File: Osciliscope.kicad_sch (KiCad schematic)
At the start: 30 parts, among them J1 USB_C_Receptacle_USB2.0_14P, U1 STM32H753VITx, X1 X322525MOB4SI

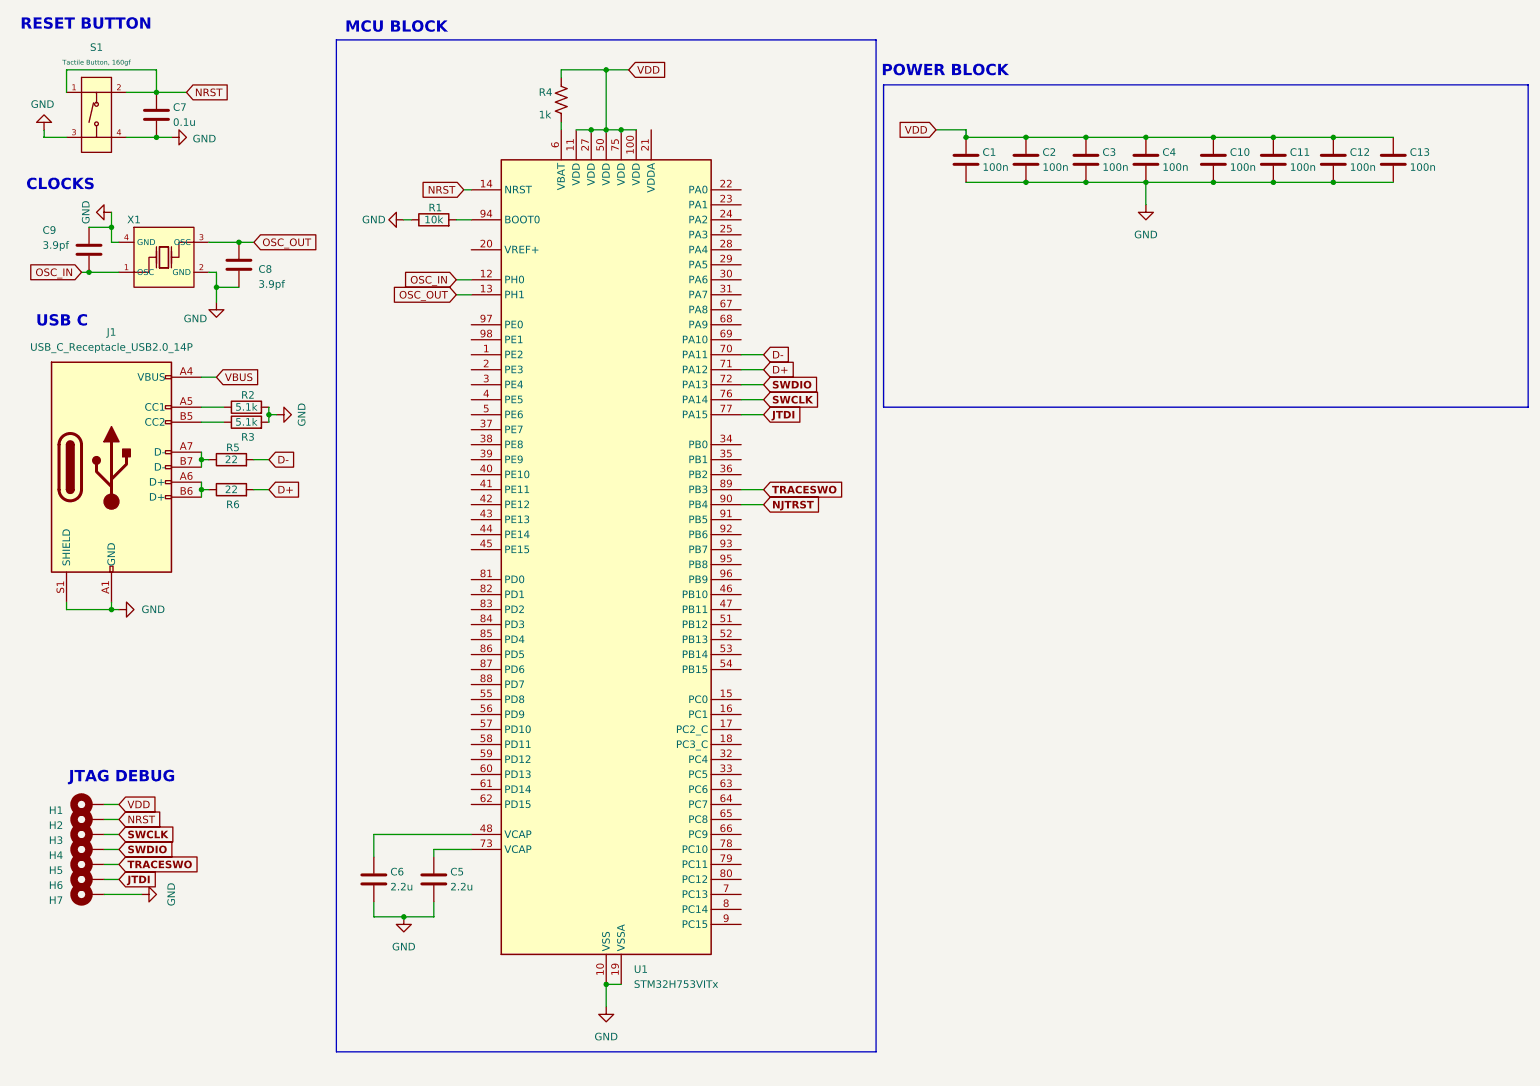
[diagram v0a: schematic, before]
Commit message: Brick all of it
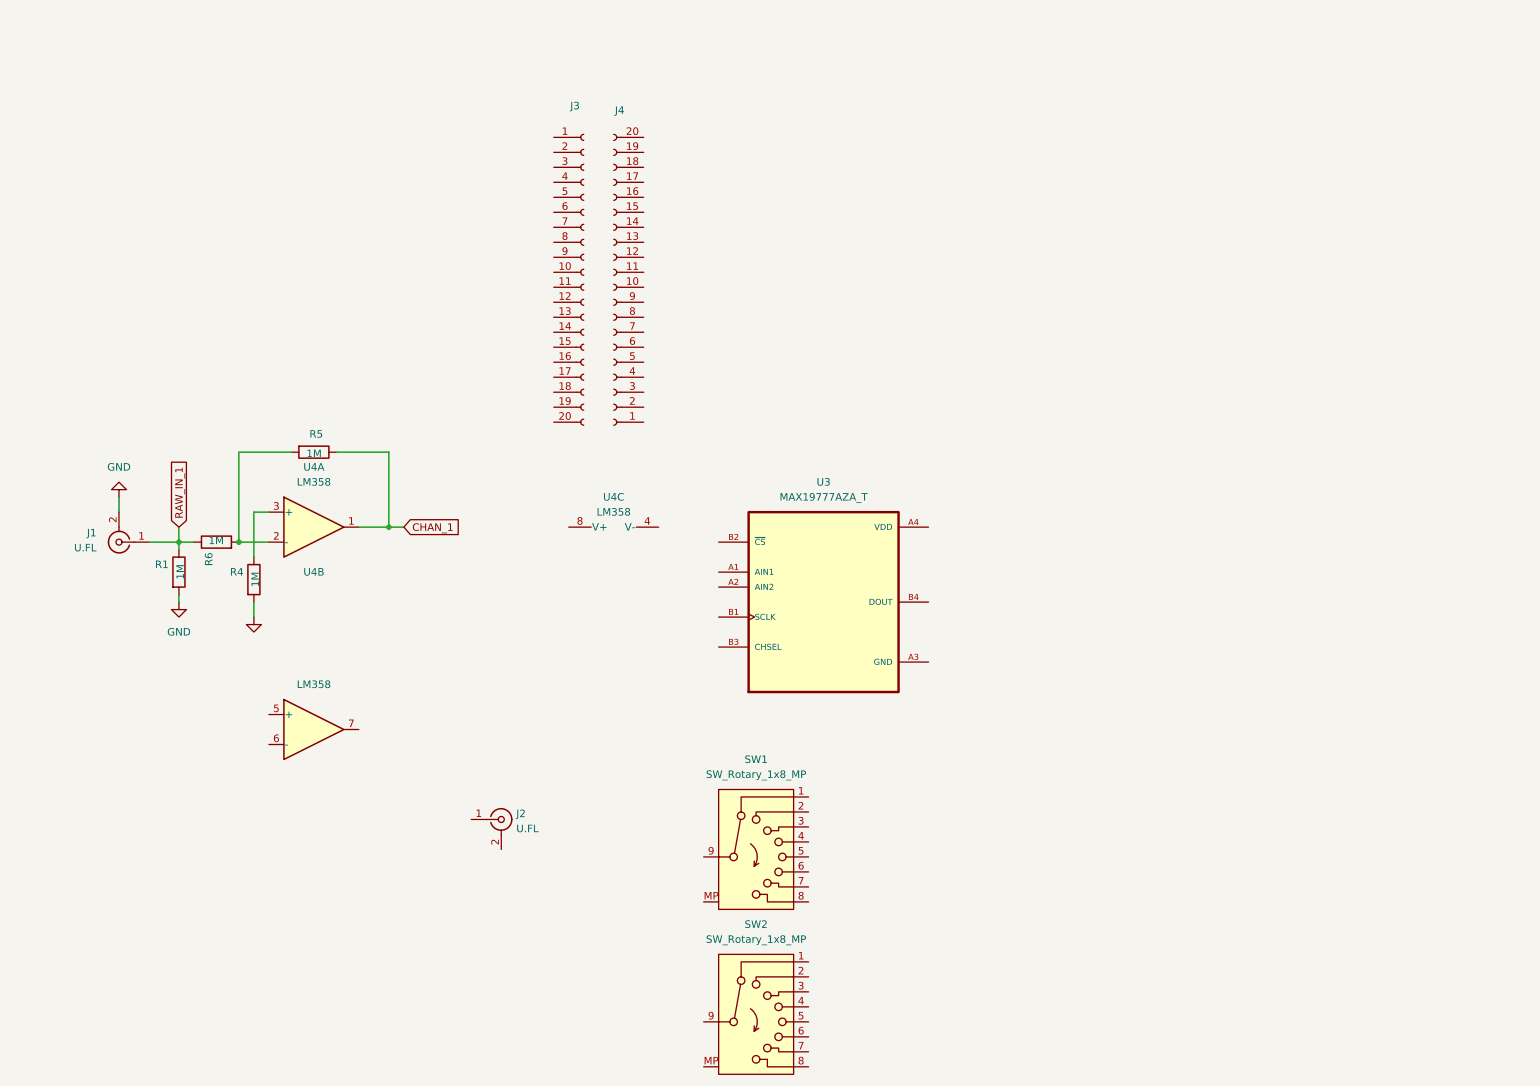
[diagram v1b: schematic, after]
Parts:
- removed C1, C10, C11, C12, C13, C2, C3, C4: 100n, symbol Device:C
- removed C5, C6: 2.2u, symbol Device:C
- removed C7: 0.1u, symbol Device:C
- removed C8, C9: 3.9pf, symbol Device:C
- removed H1, H2, H3, H4, H5, H6, H7: MountingHole_Pad, symbol Mechanical:MountingHole_Pad
- removed J1: USB_C_Receptacle_USB2.0_14P, symbol Connector:USB_C_Receptacle_USB2.0_14P
- removed R2, R3: 5.1k, symbol Device:R
- removed R4: 1k, Resistor_SMD:R_0603_1608Metric, symbol Device:R_US
- removed S1: Tactile Button, 160gf, PCM_JLCPCB:SW-SMD_4P-L5.1-W5.1-P3.70-LS6.5-TL-2, symbol PCM_JLCPCB-Connectors_Buttons:Tactile Button, 160gf, 12V, 50mA, 5.1mm
- removed U1: STM32H753VITx, Package_QFP:LQFP-100_14x14mm_P0.5mm, symbol MCU_ST_STM32H7:STM32H753VITx
- removed X1: X322525MOB4SI, PCM_JLCPCB:OSC-SMD_4P-L3.2-W2.5-BL, symbol PCM_JLCPCB-Crystals:Crystal, 25MHz, 11pF
- added J1, J2: U.FL, PCM_JLCPCB:IPEX-SMD_BWIPX-1-001E, symbol PCM_JLCPCB-Extended:RF, Connector, U.FL
- added J3, J4: Conn_01x20_Socket, symbol Connector:Conn_01x20_Socket
- added R4: 1M, symbol Device:R
- added SW1, SW2: SW_Rotary_1x8_MP, symbol Switch:SW_Rotary_1x8_MP
- added U3: MAX19777AZA_T, MAX19777AZA_T:BGA8N35P2X4_85X143X37N, symbol MAX19777AZA_T:MAX19777AZA_T
- added U4: LM358, symbol Amplifier_Operational:LM358
- R1: value 10k -> 1M
- R5, R6: value 22 -> 1M
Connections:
- net D- is gone; now on an unnamed net: R5.2
- net GND: now also R1.2, J1.2 (Ext), R4.2; no longer R1.1
- net RAW_IN_1: now reaches R6.1
- net RAW_IN_1: now also R1.1, J1.1 (In)
- net CHAN_1: now reaches R5.1
- net CHAN_1: now also U4.1
- net D+: no longer names the net of R6.2
- net D+: now also U4.2 (-)
- new net: R4.1, U4.3 (+)
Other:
- note removed: "CLOCKS"
- note removed: "JTAG DEBUG"
- note removed: "MCU BLOCK"
- note removed: "POWER BLOCK"
- note removed: "RESET BUTTON"
- note removed: "USB C"
